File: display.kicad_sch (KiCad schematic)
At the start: 22 parts, among them J3 FH34SRJ-24S-0.5SH_99_, Q1 ZXM61N03F, SW1 Button-THT - 2-1825910-7

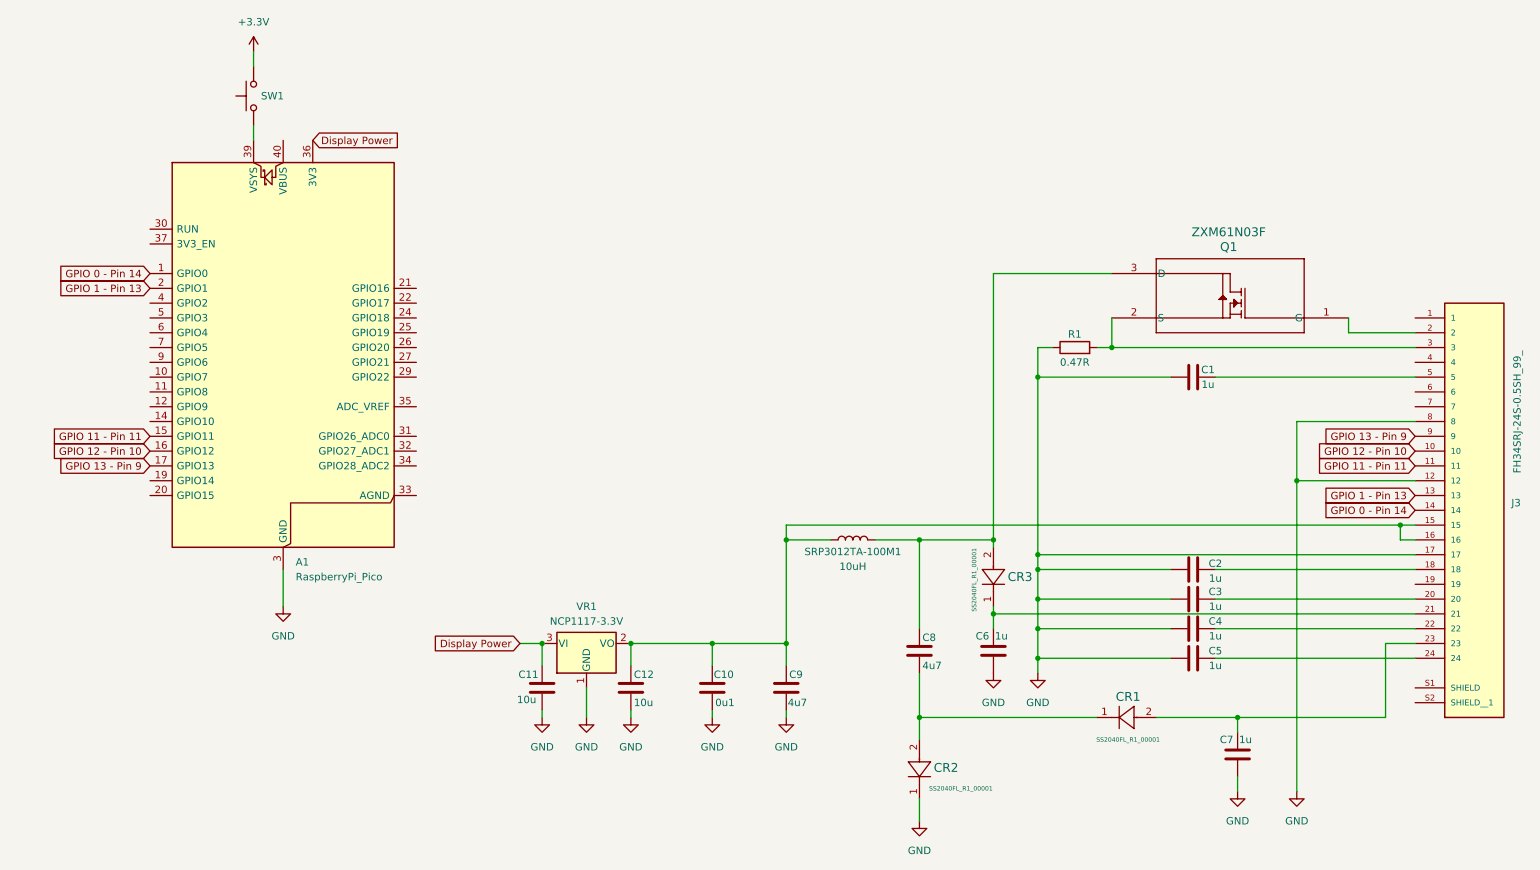
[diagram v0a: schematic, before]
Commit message: Pico connected to display (mostly???)
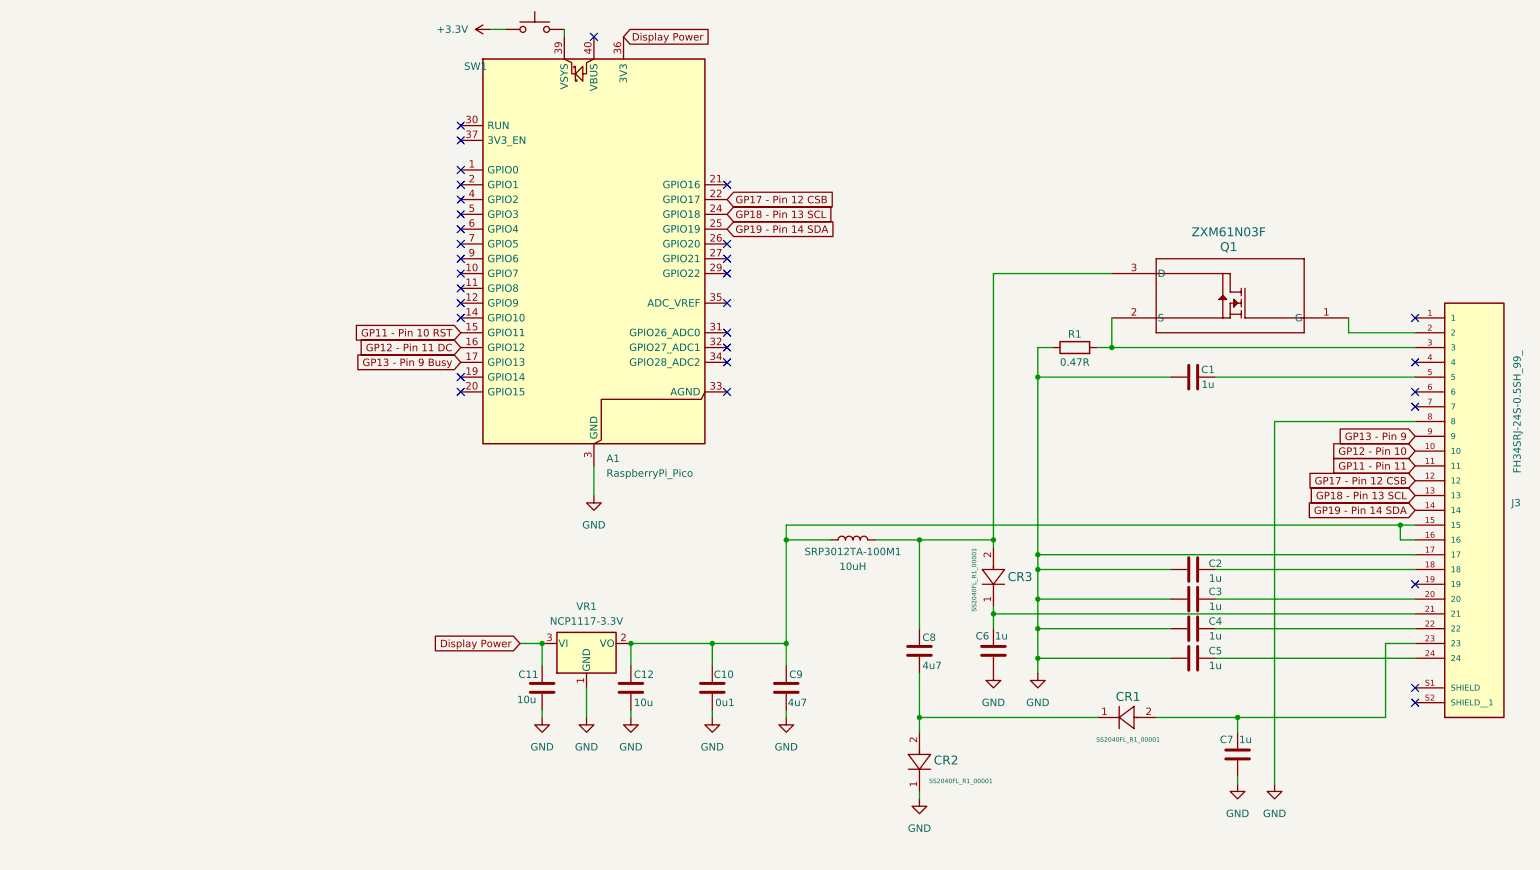
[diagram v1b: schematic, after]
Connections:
- net +3.3V: now also SW1.1; no longer SW1.2
- net GND: no longer J3.12
- net at A1.39 (VSYS): now also SW1.2; no longer SW1.1
- net GP17 - Pin 12 CSB: now reaches A1.22 (GPIO17)
- net GP17 - Pin 12 CSB: now also J3.12
- net GP18 - Pin 13 SCL: now reaches A1.24 (GPIO18)
- net GP18 - Pin 13 SCL: now also J3.13
- net GP19 - Pin 14 SDA: now reaches A1.25 (GPIO19)
- net GP19 - Pin 14 SDA: now also J3.14
- net GPIO 0 - Pin 14: no longer names the net of A1.1 (GPIO0)
- net GPIO 0 - Pin 14: no longer J3.14
- net GPIO 1 - Pin 13: no longer names the net of A1.2 (GPIO1)
- net GPIO 1 - Pin 13: no longer J3.13
- net GPIO 11 - Pin 11 renamed GP11 - Pin 10 RST
- net GP11 - Pin 10 RST: no longer J3.11
- net GPIO 12 - Pin 10 renamed GP12 - Pin 10
- net GP12 - Pin 10: no longer A1.16 (GPIO12)
- net GPIO 13 - Pin 9 renamed GP13 - Pin 9
- net GP13 - Pin 9: no longer A1.17 (GPIO13)
- new net GP11 - Pin 11: J3.11
- new net GP12 - Pin 11 DC: A1.16 (GPIO12)
- new net GP13 - Pin 9 Busy: A1.17 (GPIO13)
- no-connect marks 0 -> 32
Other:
- moved on the sheet: A1, CR2, SW1
